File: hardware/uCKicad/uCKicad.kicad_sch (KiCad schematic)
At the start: 1 part

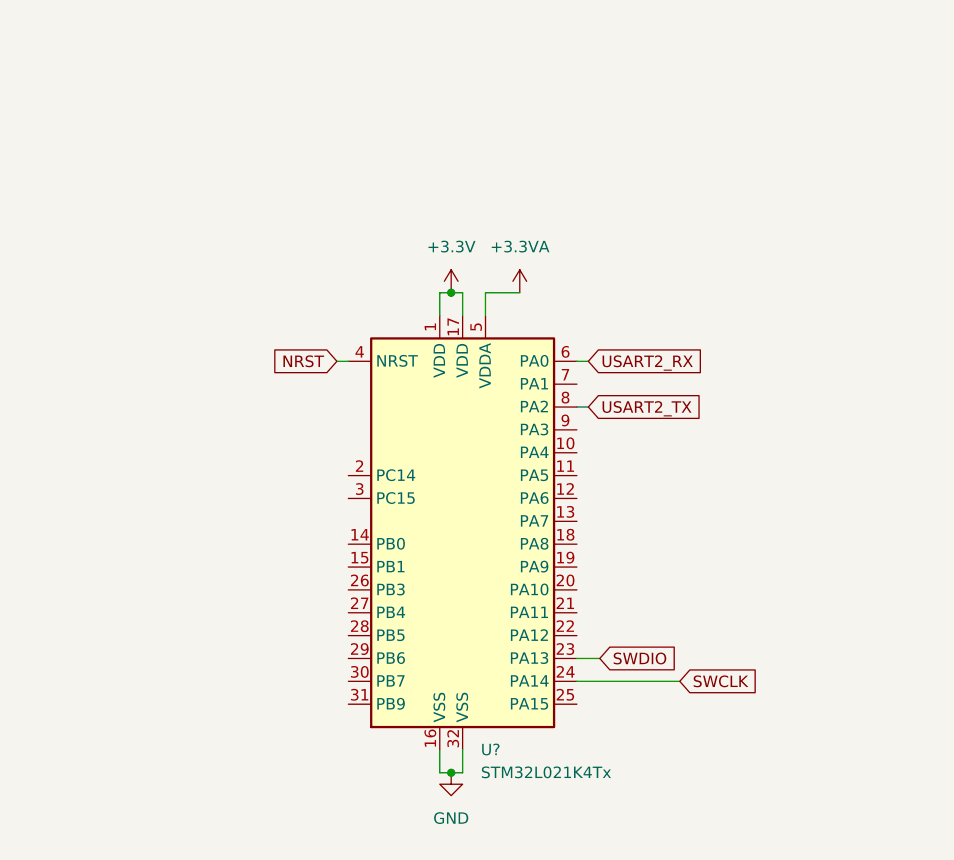
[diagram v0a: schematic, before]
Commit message: Le microcontroleur sous KiCAD part 2
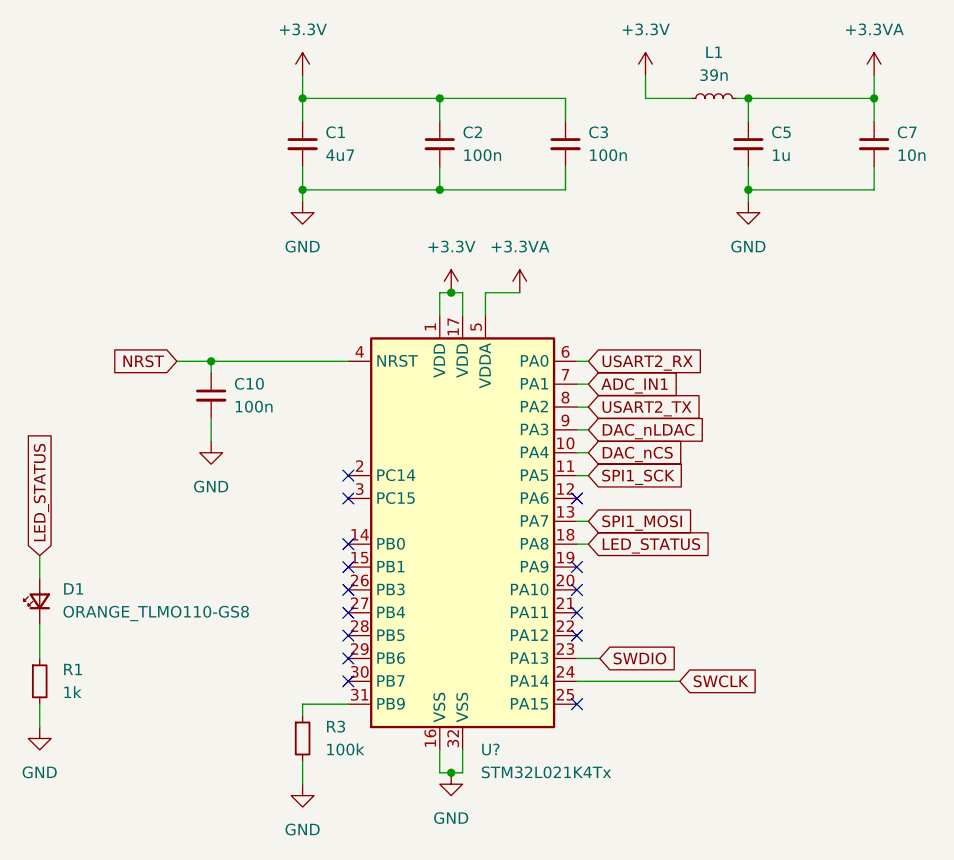
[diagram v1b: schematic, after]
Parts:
- added C1: 4u7, symbol Device:C_Small
- added C10, C2, C3: 100n, symbol Device:C_Small
- added C5: 1u, symbol Device:C_Small
- added C7: 10n, symbol Device:C_Small
- added D1: ORANGE_TLMO110-GS8, symbol Device:LED_Small
- added L1: 39n, symbol Device:L_Small
- added R1: 1k, symbol Device:R_Small
- added R3: 100k, symbol Device:R_Small
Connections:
- net +3.3V: now also C1.1, C2.1, C3.1, L1.1
- net +3.3VA: now also C5.1, C7.1, L1.2
- net GND: now also C1.2, C10.2, C2.2, C3.2, C5.2, C7.2, R1.2, R3.2
- net NRST: now also C10.1
- net DAC_nCS: now reaches U?.10 (PA4)
- net SPI1_SCK: now reaches U?.11 (PA5)
- net SPI1_MOSI: now reaches U?.13 (PA7)
- net LED_STATUS: now reaches U?.18 (PA8)
- net LED_STATUS: now also D1.2 (A)
- net at U?.31 (PB9): now also R3.1
- net ADC_IN1: now reaches U?.7 (PA1)
- net DAC_nLDAC: now reaches U?.9 (PA3)
- new net: D1.1 (K), R1.1
- no-connect marks 0 -> 15
